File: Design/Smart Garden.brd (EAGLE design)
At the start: 92 x 87 mm, 95 parts, among them IC2 MP1584EN-LF-Z, IC3 CP2102, J1 USB-C, J2 POWER_JACK, Q1 MBT3904DW1T1, T1 MMBT2222A, T3 MMBT2222A, T5 MMBT2222A, T7 MMBT2222A, U1 ESP-32S, U3 LM2596S, U4 DB107S

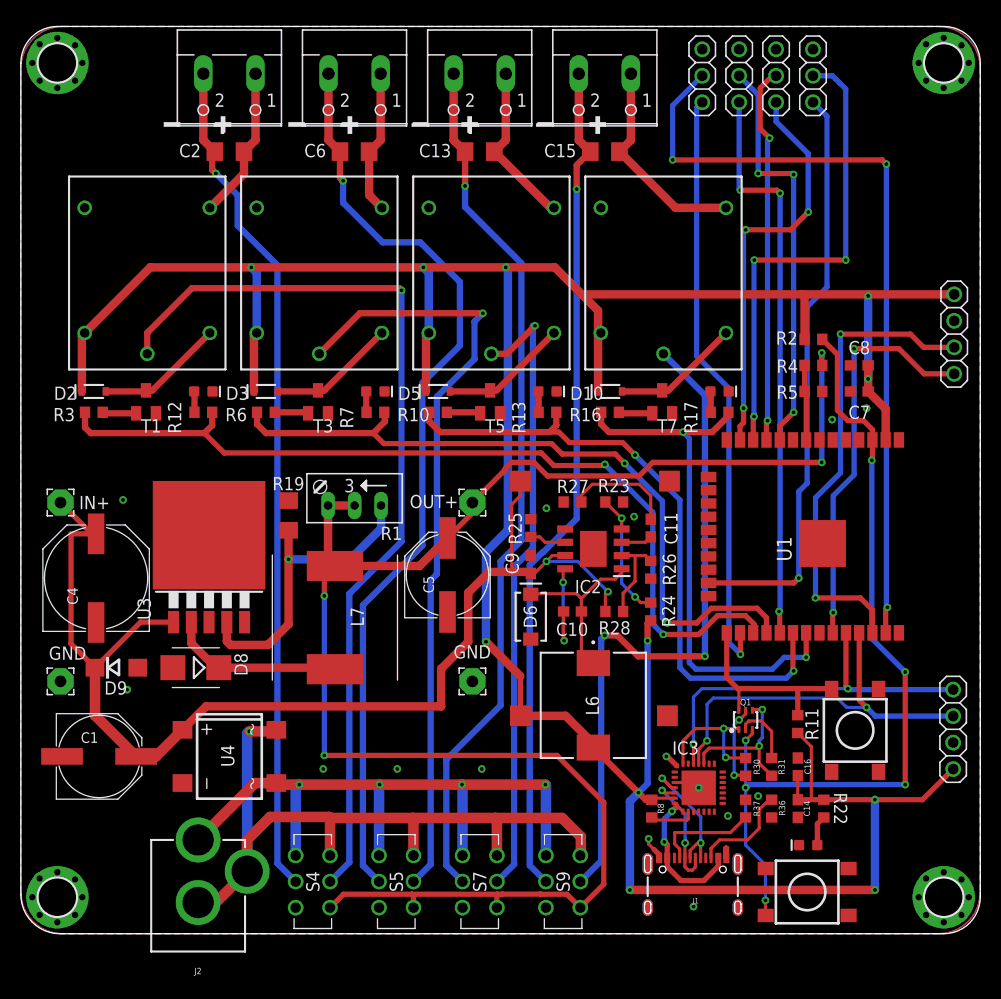
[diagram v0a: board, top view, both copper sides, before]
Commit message: Updated design files
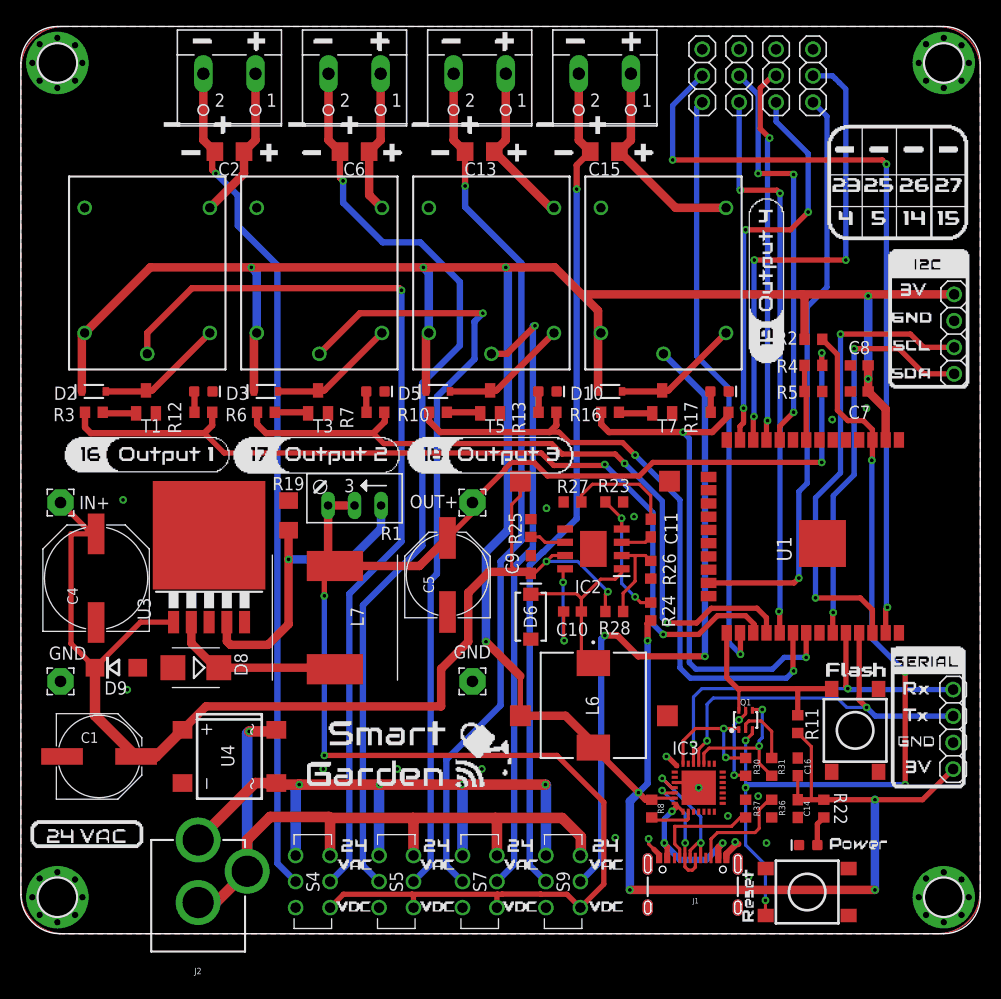
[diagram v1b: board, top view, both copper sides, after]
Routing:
- net V_USB: track 14.5 -> 15.4 mm, vias 2 -> 3
- net CC3: track 9.72 -> 10.3 mm
- net GND: track 8.15 -> 8.13 mm, vias 15 -> 18

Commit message: Updated design files
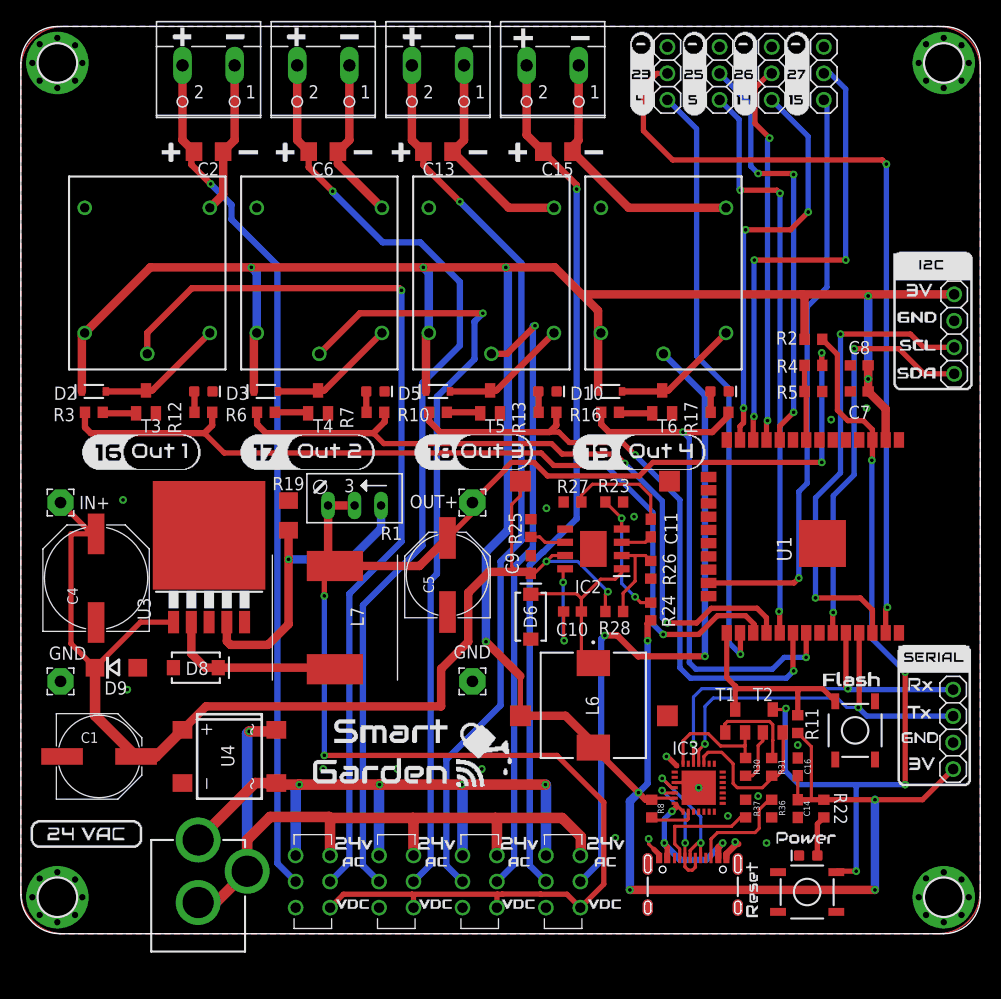
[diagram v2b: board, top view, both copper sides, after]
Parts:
- removed Q1: MBT3904DW1T1, SparkFun-DiscreteSemi:SC70-6
- added T2: MMBT3904, transistor-neu-to92:SOT23-BEC
- added T4: MMBT2222A, transistor:SOT23
- D8: value SS34 -> 3A/40V/500mV; device diode:SMB -> SparkFun-DiscreteSemi:SMA-DIODE
- D9: value RS1G -> US1M
- R23: value 40.2k -> 39k
- R24: value 124k -> 120k
- R26: value 24.9k -> 24k
- R27: value 68.1k -> 68k
- S1, S2: device Testing:TACTILE_SWITCH_TALL -> SpaceDIY_electromechanical:TACTILE_SWITCH_SMD_5.2MM
- T1: value MMBT2222A -> MMBT3904; device transistor:SOT23 -> transistor-neu-to92:SOT23-BEC
- moved T1 64.3 mm to (68.5, 20.4)
- moved T3 16.5 mm to (12.0, 51.0)
- moved X6 5.06 mm to (51.0, 82.0)
- moved C15 4.50 mm to (51.5, 75.0)
- moved X4 4.08 mm to (40.0, 82.0)
- moved C13 4.00 mm to (40.0, 75.0)
- moved JP5 3.35 mm to (62.0, 82.5)
- moved X2 3.10 mm to (29.0, 82.0)
- moved C6 3.00 mm to (29.0, 75.0)
- moved X7 2.15 mm to (18.0, 82.0)
- moved C2 2.00 mm to (18.0, 75.0)
- moved JP4 1.89 mm to (67.0, 82.5)
- moved JP2 1.07 mm to (77.0, 82.5)
- moved LED2 1.00 mm to (75.5, 7.50)
- moved JP3 0.48 mm to (72.0, 82.5)
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- renumbered T7 to T6
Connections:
- net DTR: now also T1.E; no longer Q1.1
- net ESP_RST: now also S2.3, T2.C; no longer Q1.3, S2.B2
- net GND: now also S1.1, S2.1, T4.2; no longer S1.A2, S2.A2, T1.2
- net IO0: now also S1.3, T1.C; no longer Q1.6, S1.B2
- net N$12: now also T4.3; no longer T3.3
- net N$13: now also T4.1; no longer T3.1
- net N$21: now also T2.B; no longer Q1.5
- net N$22: now also T1.B; no longer Q1.2
- net N$7: now also T3.3; no longer T1.3
- net N$9: now also T3.1; no longer T1.1
- net RTS: now also T2.E; no longer Q1.4
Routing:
- net N$52: track 20.4 -> 25.5 mm
- net N$32: track 15.9 -> 20.7 mm
- net ESP_RST: track 81.2 -> 76.6 mm, vias 6 -> 5
- net N$22: track 6.11 -> 8.91 mm
- net N$21: track 7.83 -> 5.21 mm, vias 2 -> 0
- net N$31: track 83.8 -> 86.2 mm
- net N$19: track 13.8 -> 15.9 mm
- net N$17: track 89.3 -> 91.3 mm
- net N$51: track 81.0 -> 82.8 mm
- net IO23: track 75.0 -> 76.7 mm, vias 3 -> 2
- net N$2: track 81.5 -> 83.1 mm
- net DTR: track 12.9 -> 11.4 mm, vias 2 -> 0
- net IO4: track 57.0 -> 58.1 mm
- net IO0: track 19.4 -> 20.4 mm
- net IO25: track 39.6 -> 40.6 mm
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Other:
- board text added: "JLCJLCJLCJLC"
